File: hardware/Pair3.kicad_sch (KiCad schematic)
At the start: 11 parts, among them IC2 TPS2HCS08AQPWPRQ1, J14 Conn_01x02, J6 Conn_01x02

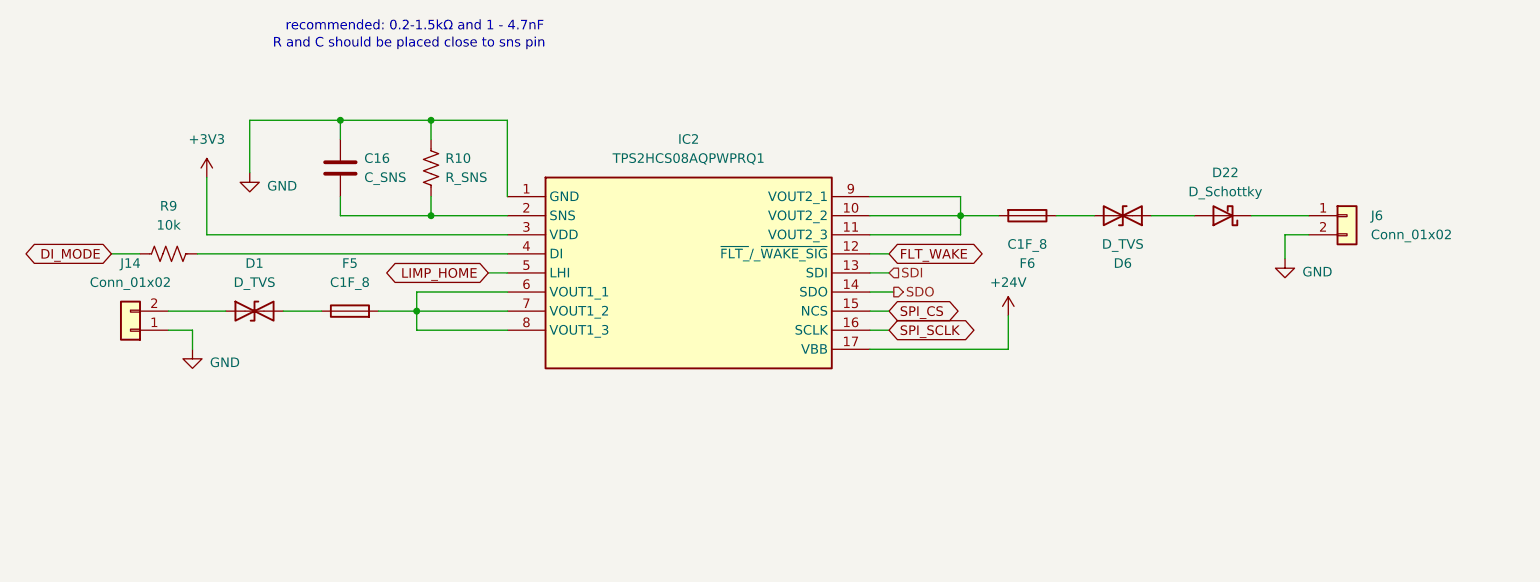
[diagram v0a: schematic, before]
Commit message: aesthetic added
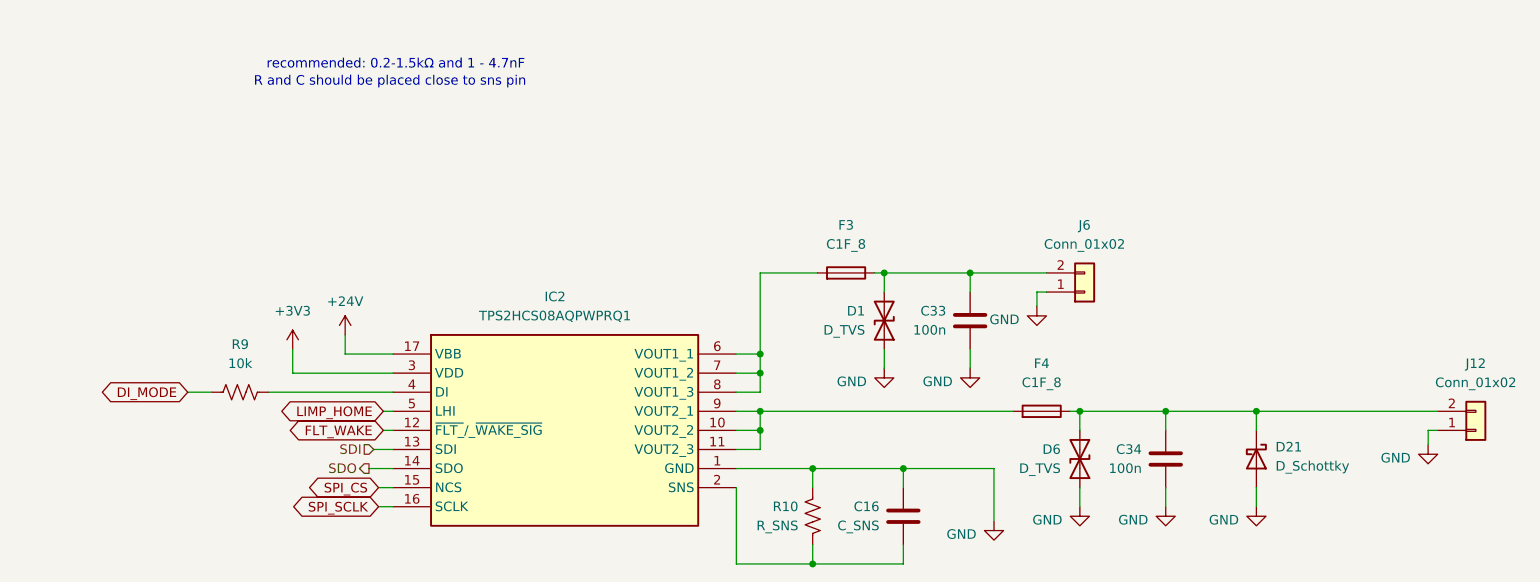
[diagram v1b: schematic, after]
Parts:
- removed D22: D_Schottky, symbol Device:D_Schottky
- removed F5, F6: C1F_8, Fuse:Fuse_1206_3216Metric, symbol PowerDistributionUnitLib:C1F_8
- removed J14: Conn_01x02, symbol Connector_Generic:Conn_01x02
- added C33, C34: 100n, symbol Device:C
- added D21: D_Schottky, symbol Device:D_Schottky
- added F3, F4: C1F_8, Fuse:Fuse_1206_3216Metric, symbol PowerDistributionUnitLib:C1F_8
- added J12: Conn_01x02, symbol Connector_Generic:Conn_01x02
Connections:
- net GND: now also D1.1 (A1), D6.1 (A1), J6.1 (Pin_1), C33.1, C34.1, D21.2 (A), J12.1 (Pin_1); no longer J6.2 (Pin_2)
- net at D6.2 (A2): now also C34.2, D21.1 (K), F4.1, J12.2 (Pin_2)
- net at IC2.10 (VOUT2_2), IC2.11 (VOUT2_3), IC2.9 (VOUT2_1): now also F4.2
- net at IC2.6 (VOUT1_1), IC2.7 (VOUT1_2), IC2.8 (VOUT1_3): now also F3.2
- net at D1.2 (A2): now also J6.2 (Pin_2), C33.2, F3.1
